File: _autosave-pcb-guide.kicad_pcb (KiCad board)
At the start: 2 copper layers, 24 parts, among them SW1 SW_Push, U1 ATmega32U4-AU, Y1 16Mhz

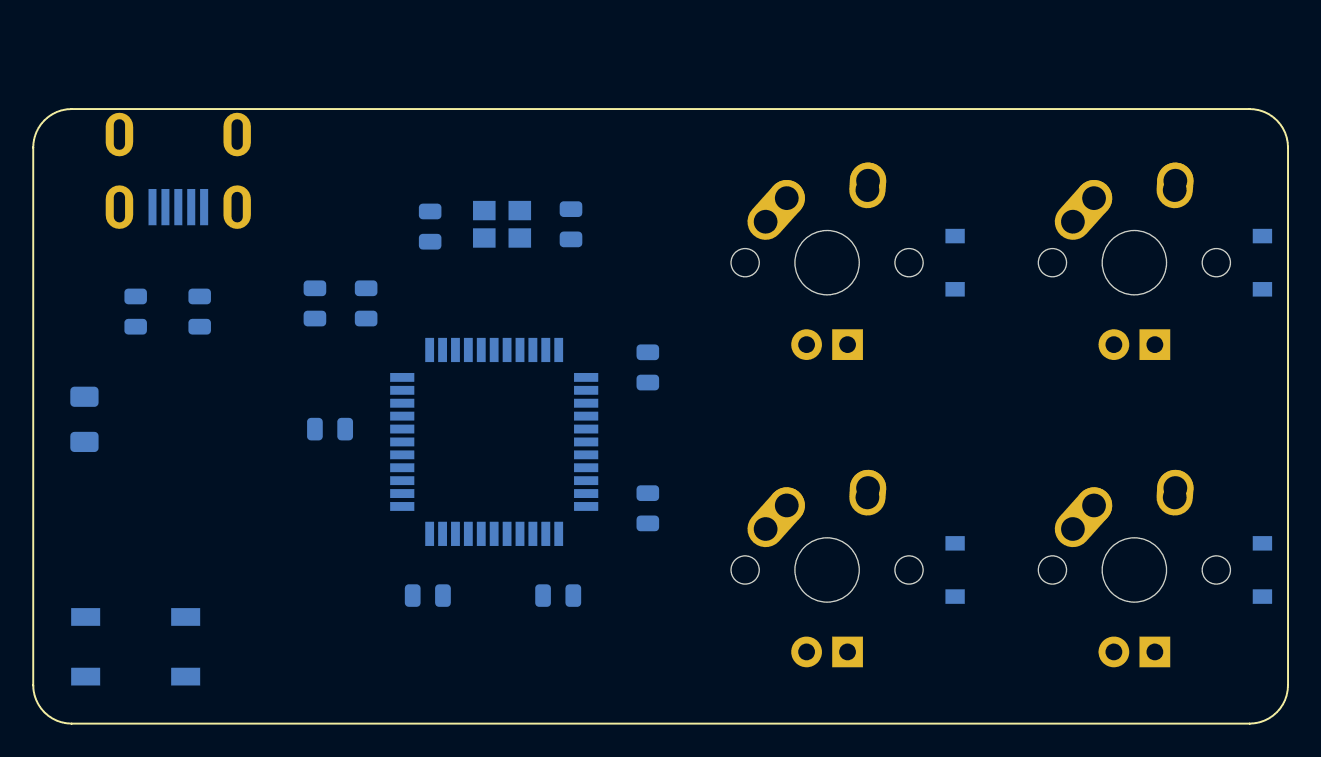
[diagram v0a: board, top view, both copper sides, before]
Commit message: PCB finished
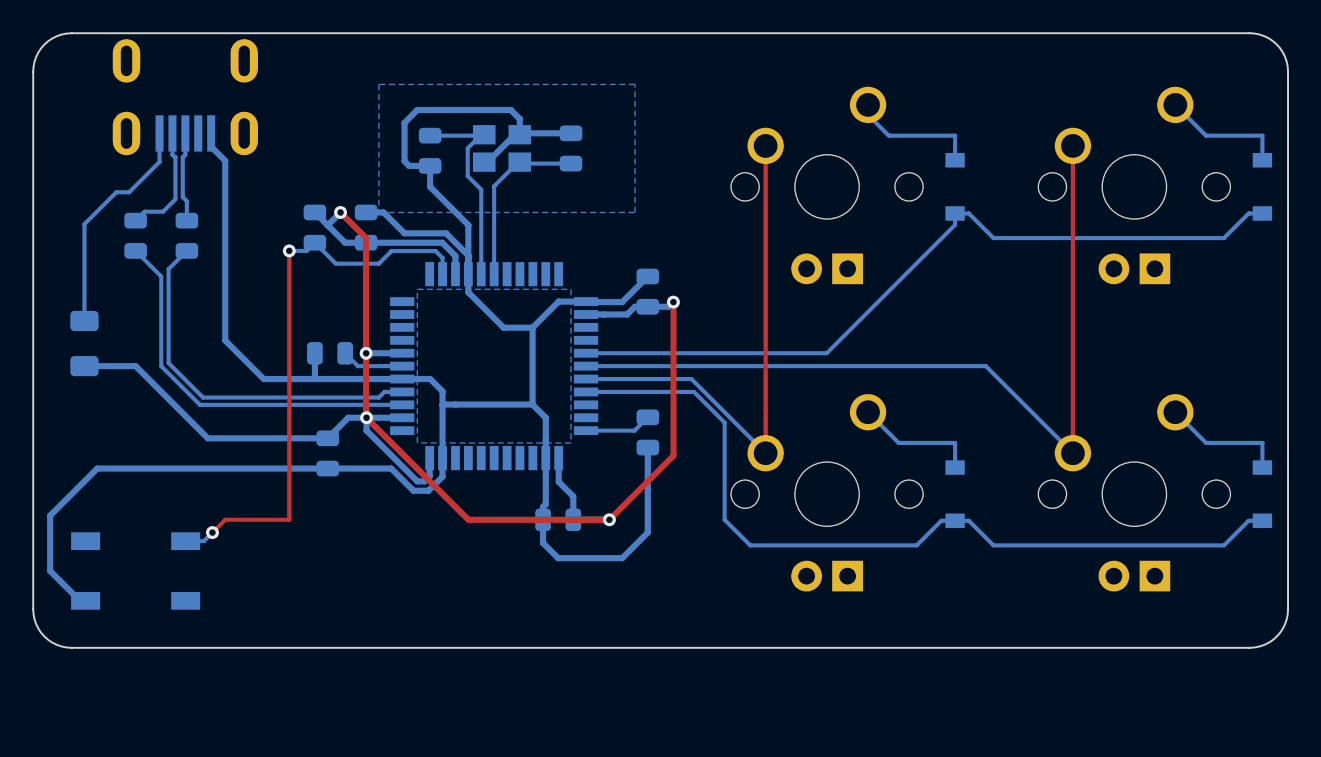
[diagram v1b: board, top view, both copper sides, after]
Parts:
- MX1, MX2, MX3, MX4: footprint MX_Alps_Hybrid:MX-1U -> MX_Only:MXOnly-1U
- moved C7 10.8 mm to (183.4, 51.5), turned to 270 degrees
- moved R2 4.77 mm to (174.6, 38.0)
- moved C2 4.70 mm to (189.7, 32.8)
- moved C6 4.70 mm to (197.6, 55.6)
- moved C1 4.70 mm to (198.4, 32.6)
- moved C3 4.70 mm to (183.5, 45.3)
- moved C4 4.70 mm to (185.7, 37.5)
- moved C5 4.70 mm to (203.2, 41.5)
- moved D1 4.70 mm to (222.2, 35.0)
- moved D2 4.70 mm to (241.3, 35.0)
- moved D3 4.70 mm to (222.2, 54.0)
- moved D4 4.70 mm to (241.3, 54.0)
- moved F1 4.70 mm to (168.3, 44.7), turned to 90 degrees
- moved MX1 4.70 mm to (214.3, 35.0)
- moved MX2 4.70 mm to (233.4, 35.0)
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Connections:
- U1 pad 1: Net-(U1-Pad1) -> (no net)
- U1 pad 10: Net-(U1-Pad10) -> (no net)
- U1 pad 11: Net-(U1-Pad11) -> (no net)
- U1 pad 12: Net-(U1-Pad12) -> (no net)
- U1 pad 18: Net-(U1-Pad18) -> (no net)
- U1 pad 19: Net-(U1-Pad19) -> (no net)
- U1 pad 20: Net-(U1-Pad20) -> (no net)
- U1 pad 21: Net-(U1-Pad21) -> (no net)
- U1 pad 22: Net-(U1-Pad22) -> (no net)
- U1 pad 25: Net-(U1-Pad25) -> (no net)
- U1 pad 26: Net-(U1-Pad26) -> (no net)
- U1 pad 27: Net-(U1-Pad27) -> ROW0
- U1 pad 28: Net-(U1-Pad28) -> COL1
- U1 pad 29: Net-(U1-Pad29) -> COL0
- U1 pad 30: Net-(U1-Pad30) -> ROW1
- U1 pad 31: Net-(U1-Pad31) -> (no net)
- U1 pad 32: Net-(U1-Pad32) -> (no net)
- U1 pad 36: Net-(U1-Pad36) -> (no net)
- U1 pad 37: Net-(U1-Pad37) -> (no net)
- U1 pad 38: Net-(U1-Pad38) -> (no net)
- U1 pad 39: Net-(U1-Pad39) -> (no net)
- U1 pad 40: Net-(U1-Pad40) -> (no net)
- U1 pad 41: Net-(U1-Pad41) -> (no net)
- U1 pad 42: Net-(U1-Pad42) -> (no net)
- U1 pad 8: Net-(U1-Pad8) -> (no net)
- U1 pad 9: Net-(U1-Pad9) -> (no net)
- USB1 pad 2: Net-(USB1-Pad2) -> (no net)
- USB1 pad 3: Net-(USB1-Pad3) -> D+
- USB1 pad 4: D+ -> D-
- USB1 pad 5: D- -> VCC
- USB1 pad 6: VCC -> Net-(USB1-Pad6)
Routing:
- net GND: track 0.00 -> 149.9 mm
- net +5V: track 0.00 -> 102.6 mm, vias 0 -> 5
- net COL1: track 0.00 -> 51.5 mm, vias 0 -> 1
- net ROW1: track 0.00 -> 51.3 mm
- net ROW0: track 0.00 -> 47.2 mm
- net Net-(R1-Pad2): track 0.00 -> 35.4 mm, vias 0 -> 2
- net COL0: track 0.00 -> 32.1 mm, vias 0 -> 3
- net Net-(R3-Pad1): track 0.00 -> 23.7 mm
- net Net-(R2-Pad1): track 0.00 -> 22.9 mm
- net VCC: track 0.00 -> 14.1 mm
- net Net-(C2-Pad1): track 0.00 -> 12.9 mm
- net Net-(C1-Pad1): track 0.00 -> 10.9 mm
- net Net-(D3-Pad2): track 0.00 -> 7.86 mm
- net Net-(D4-Pad2): track 0.00 -> 7.71 mm
- net Net-(D1-Pad2): track 0.00 -> 7.51 mm
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- added copper zone on B.Cu, net GND
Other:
- board outline added: 77.8 x 38.1 mm
- net class Default: trace_width 0.25 -> 0.254
- net class Power added: clearance 0.2, trace_width 0.381, via_dia 0.8, via_drill 0.4
- rule trace_min: 0.2 -> 0
